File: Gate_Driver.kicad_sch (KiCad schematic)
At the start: 27 parts, among them U1 DRV8323RSRGZR

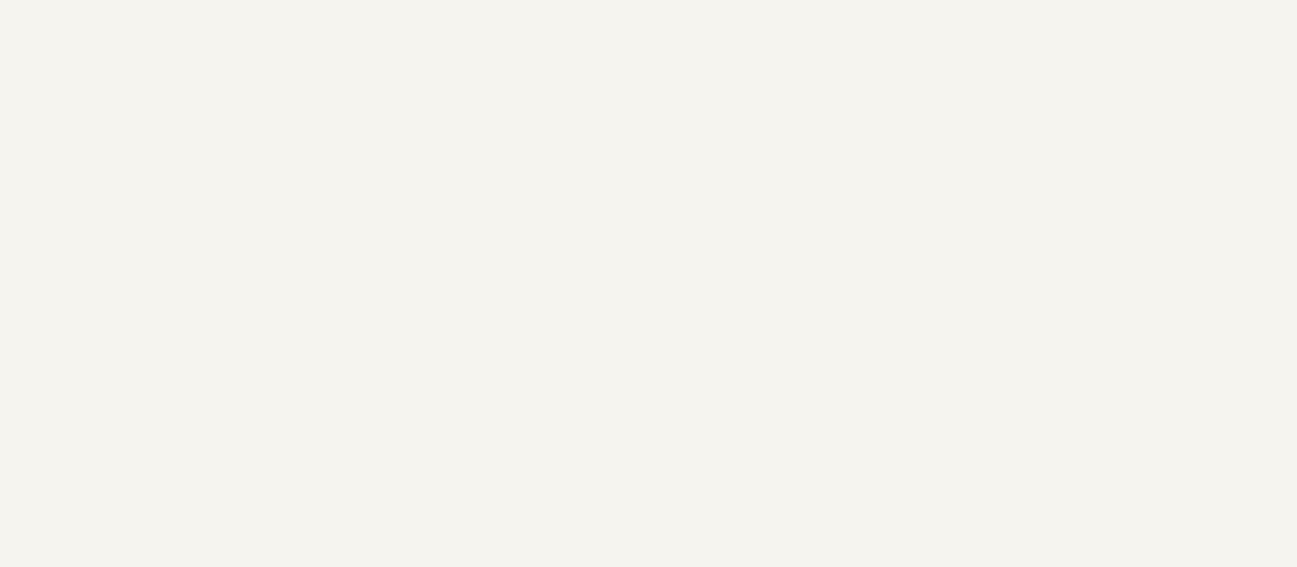
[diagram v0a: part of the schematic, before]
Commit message: nothing
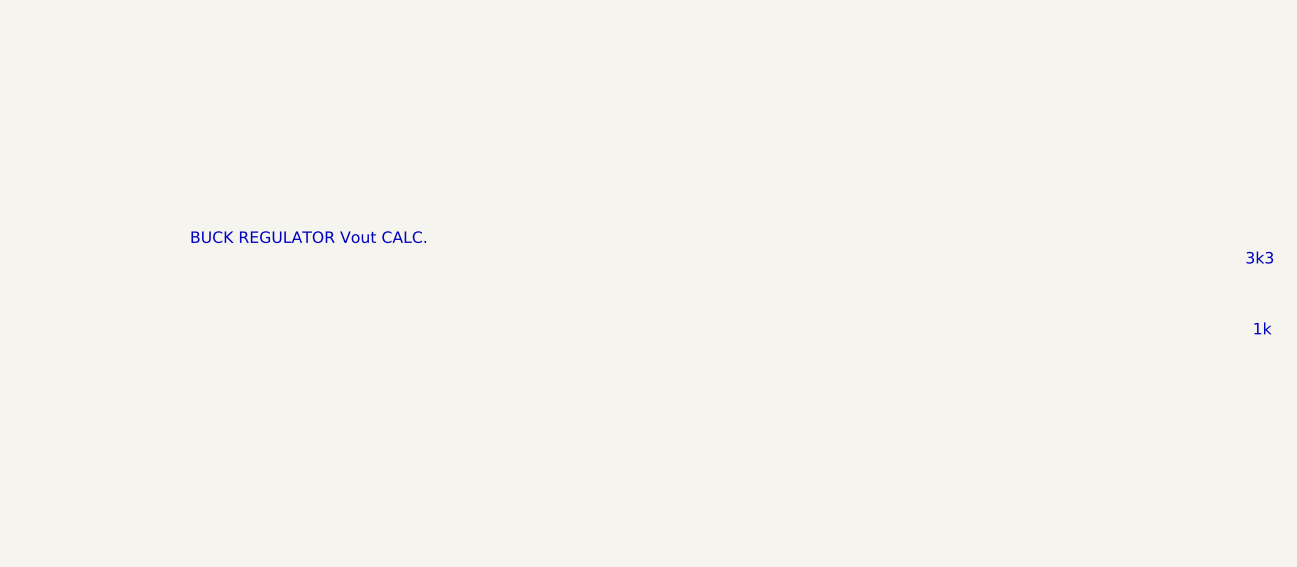
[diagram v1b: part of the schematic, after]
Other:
- note added: "1k"
- note added: "3k3"
- note added: "BUCK REGULATOR Vout CALC."

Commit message: Revert "nothing"
This reverts commit c8bc8ca9c45f61fe26da700702173eff74c7b1f5.
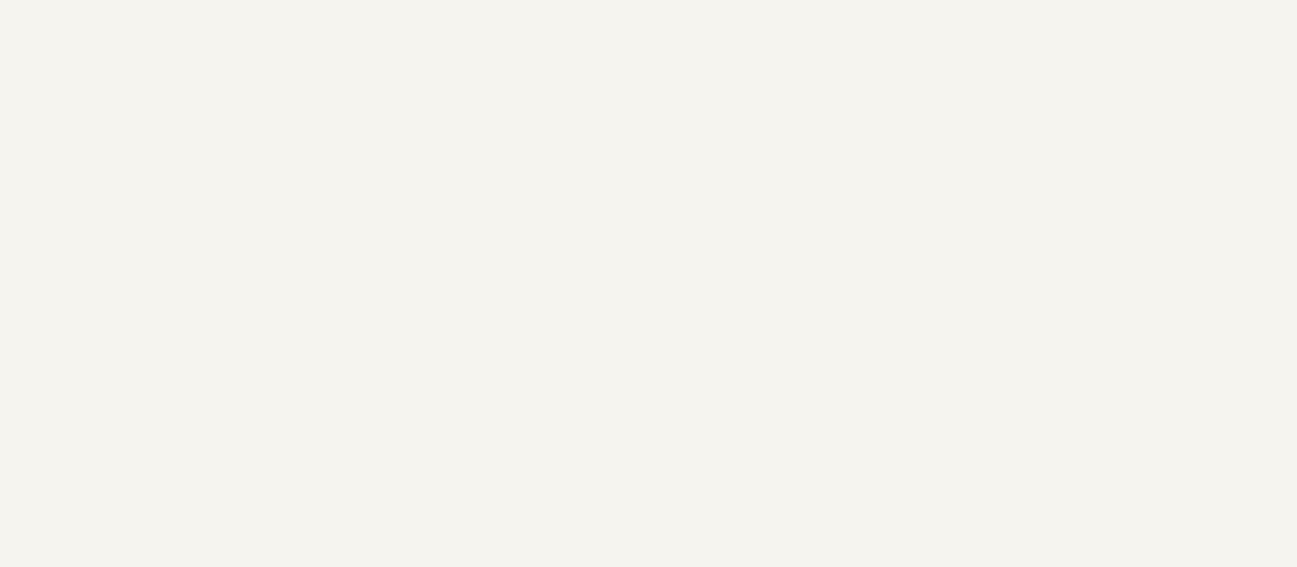
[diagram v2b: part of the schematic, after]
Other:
- note removed: "1k"
- note removed: "3k3"
- note removed: "BUCK REGULATOR Vout CALC."
